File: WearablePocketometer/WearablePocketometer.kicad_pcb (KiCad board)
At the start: 2 copper layers, 66 x 66 mm, 97 parts, among them J101 SolderJumper_2_Bridged, J102 Conn_02x06_Male, J107 SolderJumper_2_Bridged, J111 SolderJumper_2_Bridged, J112 Conn_02x06_Male, J117 SolderJumper_2_Bridged, J120 STANDOFF, J1201 Conn_01x09_Male, J1202 SolderJumper_2_Bridged, J1207 SolderJumper_2_Bridged, J125 STANDOFF, J127 STANDOFF, J129 STANDOFF, J1601 USB_C_Receptacle_USB2.0, J201 SolderJumper_2_Open, J202 Conn_02x06_Male, J207 SolderJumper_2_Open, J701 USB_C_Receptacle_USB2.0, U1001 LSM6DSO, U101 AK09970, U102 P82B96, U104 Teensy4.1, U1101 BME280, U112 P82B96, U1201 AK09970, U1202 P82B96, U1301 LSM6DSO, U1401 BME280, U1501 LSM6DSO, U201 AK09970, U202 P82B96, U301 LSM6DSO, U401 BME280, U501 LSM6DSO, U601 NEO_M8U, U701 USBLC6-2SC6, U801 MIC5319 3.3V, U901 LSM6DSO, Y601 W3011

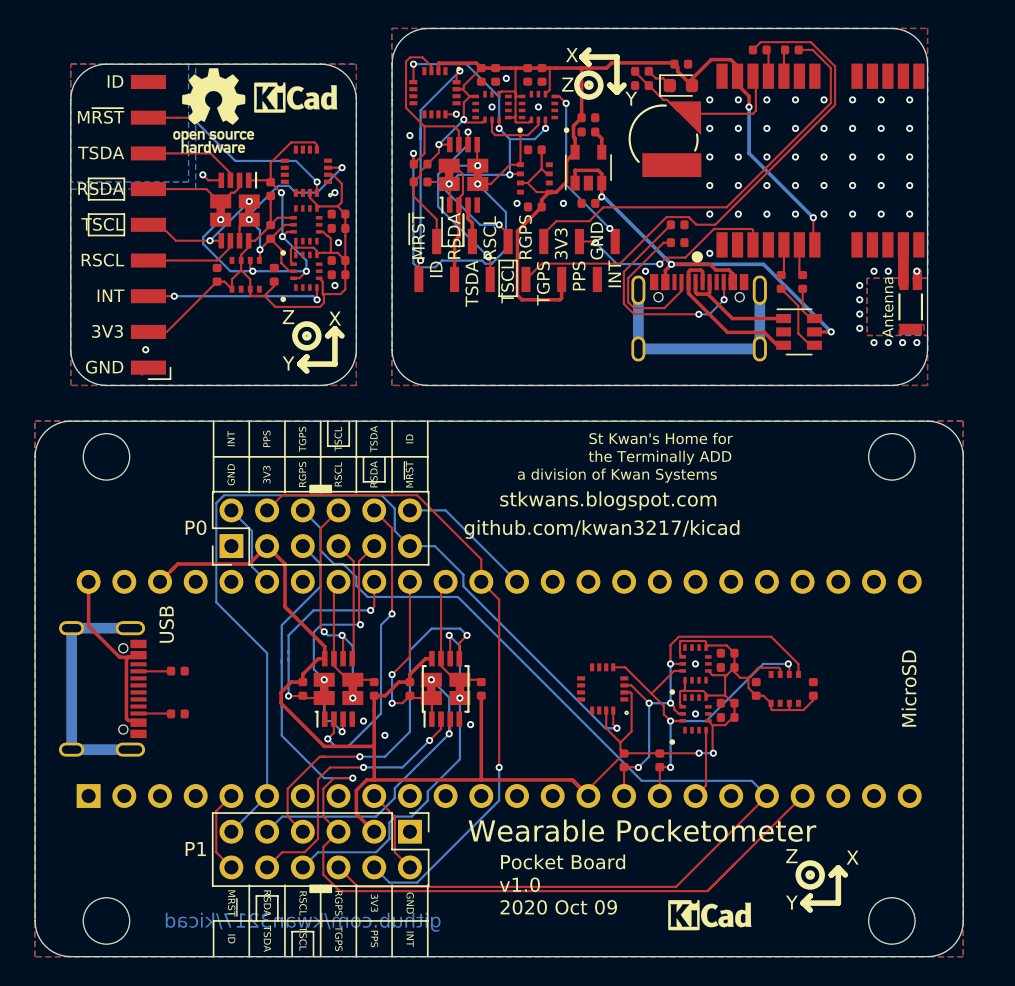
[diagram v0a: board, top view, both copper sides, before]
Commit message: j
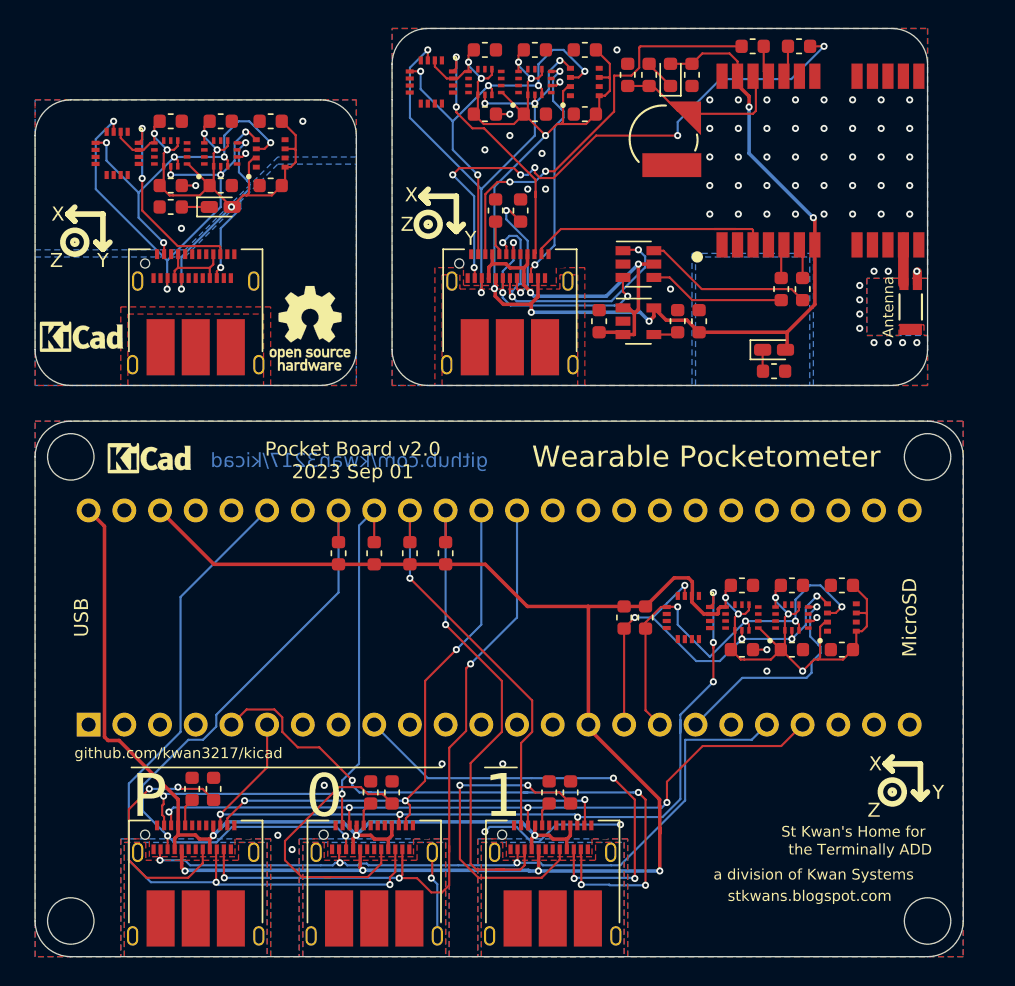
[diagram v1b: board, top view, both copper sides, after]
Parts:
- removed the C801 at (113.0, 73.4)
- removed C804: 100nF, Capacitor_SMD:C_0402_1005Metric
- removed C805: 2.2uF, Capacitor_SMD:C_0402_1005Metric
- removed the G101 at (80.5, 96.3)
- removed the J102 at (100.3, 118.1)
- removed J107, J111, J117, J1202, J1207: SolderJumper_2_Bridged, KwanSystems:SolderJumper-2_Bridged
- removed J112: Conn_02x06_Male, Connector_PinHeader_2.54mm:PinHeader_2x06_P2.54mm_Vertical
- removed J120: STANDOFF, KwanSystems:STANDOFF_NONPLATED
- removed J1601, J701: USB_C_Receptacle_USB2.0, KwanSystems:GCTUSBTypeC_PTH
- removed J201, J207: SolderJumper_2_Open, KwanSystems:SolderJumper-2_Bridged
- removed J202: Conn_02x06_Male, Connector_PinSocket_1.27mm:PinSocket_1x12_P1.27mm_Vertical_SMD_Pin1Left
- removed R1207, R201, R207: 10k, Resistor_SMD:R_0402_1005Metric
- removed R1601, R1602, R701, R702: 5.1k, Resistor_SMD:R_0402_1005Metric
- removed U104: Teensy4.1, KwanSystems:Teensy2x24
- removed U112, U1202, U202: P82B96, Package_SO:TSSOP-8_3x3mm_P0.65mm
- removed the U701 at (128.0, 82.5)
- removed the U801 at (113.0, 70.9)
- added C1001: 1uF, Capacitor_SMD:C_0603_1608Metric, F.Cu at (113.8, 81.8)
- added C1002: 100nF, Capacitor_SMD:C_0603_1608Metric, F.Cu at (119.4, 81.8)
- added C1003: 2.2uF, Capacitor_SMD:C_0603_1608Metric, F.Cu at (120.9, 81.8)
- added D1301: RED, LED_SMD:LED_0603_1608Metric_Castellated, F.Cu at (86.9, 73.7)
- added D501: RED, LED_SMD:LED_0603_1608Metric_Castellated, F.Cu at (126.2, 83.8)
- added J1101: USB_C_Receptacle, KwanSystems:USB_C_Receptacle_Amphenol_12401610E4-2A, F.Cu at (110.5, 122.7)
- added J1701: USB_C_Receptacle, KwanSystems:USB_C_Receptacle_Amphenol_12401610E4-2A, F.Cu at (97.8, 122.7)
- added J1801: USB_C_Receptacle, KwanSystems:USB_C_Receptacle_Amphenol_12401610E4-2A, F.Cu at (85.1, 82.0)
- added J1901: USB_C_Receptacle, KwanSystems:USB_C_Receptacle_Amphenol_12401610E4-2A, F.Cu at (85.1, 122.7)
- added R1101: 5.1k, Resistor_SMD:R_0603_1608Metric, F.Cu at (110.2, 115.3)
- added R1102: 5.1k, Resistor_SMD:R_0603_1608Metric, F.Cu at (111.8, 115.3)
- added R1202: 5.1k, Resistor_SMD:R_0603_1608Metric, F.Cu at (108.2, 73.9)
- added R1301: 1k, Resistor_SMD:R_0603_1608Metric, F.Cu at (83.3, 73.7)
- added R1701: 5.1k, Resistor_SMD:R_0603_1608Metric, F.Cu at (97.5, 115.3)
- added R1702: 5.1k, Resistor_SMD:R_0603_1608Metric, F.Cu at (99.1, 115.3)
- added R1901: 5.1k, Resistor_SMD:R_0603_1608Metric, F.Cu at (84.8, 115.1)
- added R1902: 5.1k, Resistor_SMD:R_0603_1608Metric, F.Cu at (86.4, 115.1)
- added R501: 1k, Resistor_SMD:R_0603_1608Metric, F.Cu at (126.2, 85.3)
- added U1001: MIC5319 3.3V, Package_TO_SOT_SMD:SOT-23-5, F.Cu at (116.6, 81.8)
- added U1201: USBLC6-2SC6, Package_TO_SOT_SMD:SOT-23-6, F.Cu at (116.6, 77.7)
- C1401: renamed from C1305; footprint Capacitor_SMD:C_0402_1005Metric -> Capacitor_SMD:C_0603_1608Metric
- C1402: renamed from C1308; footprint Capacitor_SMD:C_0402_1005Metric -> Capacitor_SMD:C_0603_1608Metric
- C1501: renamed from C1406; footprint Capacitor_SMD:C_0402_1005Metric -> Capacitor_SMD:C_0603_1608Metric
- C1502: renamed from C1408; footprint Capacitor_SMD:C_0402_1005Metric -> Capacitor_SMD:C_0603_1608Metric
- C1601: renamed from C1505; footprint Capacitor_SMD:C_0402_1005Metric -> Capacitor_SMD:C_0603_1608Metric
- C1602: renamed from C1508; footprint Capacitor_SMD:C_0402_1005Metric -> Capacitor_SMD:C_0603_1608Metric
- C201: renamed from C905; footprint Capacitor_SMD:C_0402_1005Metric -> Capacitor_SMD:C_0603_1608Metric
- C202: renamed from C908; footprint Capacitor_SMD:C_0402_1005Metric -> Capacitor_SMD:C_0603_1608Metric
- C301: renamed from C1005; footprint Capacitor_SMD:C_0402_1005Metric -> Capacitor_SMD:C_0603_1608Metric
- C302: renamed from C1008; footprint Capacitor_SMD:C_0402_1005Metric -> Capacitor_SMD:C_0603_1608Metric
- C401: renamed from C1106; footprint Capacitor_SMD:C_0402_1005Metric -> Capacitor_SMD:C_0603_1608Metric
- C402: renamed from C1108; footprint Capacitor_SMD:C_0402_1005Metric -> Capacitor_SMD:C_0603_1608Metric
- C601: renamed from C305; footprint Capacitor_SMD:C_0402_1005Metric -> Capacitor_SMD:C_0603_1608Metric
- C602: renamed from C308; footprint Capacitor_SMD:C_0402_1005Metric -> Capacitor_SMD:C_0603_1608Metric
- C701: renamed from C406; footprint Capacitor_SMD:C_0402_1005Metric -> Capacitor_SMD:C_0603_1608Metric
- C702: renamed from C408; footprint Capacitor_SMD:C_0402_1005Metric -> Capacitor_SMD:C_0603_1608Metric
- C801: renamed from C505; footprint Capacitor_SMD:C_0402_1005Metric -> Capacitor_SMD:C_0603_1608Metric
- C802: renamed from C508; footprint Capacitor_SMD:C_0402_1005Metric -> Capacitor_SMD:C_0603_1608Metric
- C901: renamed from C601; footprint Capacitor_SMD:C_0402_1005Metric -> Capacitor_SMD:C_0603_1608Metric
- G104: renamed from G103; moved to F.Cu
- J101: value SolderJumper_2_Bridged -> STANDOFF; footprint KwanSystems:SolderJumper-2_Bridged -> KwanSystems:STANDOFF_NONPLATED
- J1201: value Conn_01x09_Male -> USB_C_Receptacle; footprint Connector_Harwin:Harwin_M20-89009xx_1x09_P2.54mm_Horizontal -> KwanSystems:USB_C_Receptacle_Amphenol_12401610E4-2A
- R101: renamed from R117; value 10k -> 1k; footprint Resistor_SMD:R_0402_1005Metric -> Resistor_SMD:R_0603_1608Metric
- R102: renamed from R116; value 10k -> 1k; footprint Resistor_SMD:R_0402_1005Metric -> Resistor_SMD:R_0603_1608Metric
- R103: renamed from R141; value 10k -> 1k; footprint Resistor_SMD:R_0402_1005Metric -> Resistor_SMD:R_0603_1608Metric
- R104: renamed from R140; value 10k -> 1k; footprint Resistor_SMD:R_0402_1005Metric -> Resistor_SMD:R_0603_1608Metric
- R105: renamed from R139; value 10k -> 1k; footprint Resistor_SMD:R_0402_1005Metric -> Resistor_SMD:R_0603_1608Metric
- R106: renamed from R138; value 10k -> 1k; footprint Resistor_SMD:R_0402_1005Metric -> Resistor_SMD:R_0603_1608Metric
- R1201: value 10k -> 5.1k; footprint Resistor_SMD:R_0402_1005Metric -> Resistor_SMD:R_0603_1608Metric
- R901: renamed from R605; footprint Resistor_SMD:R_0402_1005Metric -> Resistor_SMD:R_0603_1608Metric
- R902: renamed from R606; footprint Resistor_SMD:R_0402_1005Metric -> Resistor_SMD:R_0603_1608Metric
- R903: renamed from R602; footprint Resistor_SMD:R_0402_1005Metric -> Resistor_SMD:R_0603_1608Metric
- R904: renamed from R603; footprint Resistor_SMD:R_0402_1005Metric -> Resistor_SMD:R_0603_1608Metric
- R905: renamed from R621; footprint Resistor_SMD:R_0402_1005Metric -> Resistor_SMD:R_0603_1608Metric
- R906: renamed from R620; footprint Resistor_SMD:R_0402_1005Metric -> Resistor_SMD:R_0603_1608Metric
- U102: value P82B96 -> Teensy4.1; footprint Package_SO:TSSOP-8_3x3mm_P0.65mm -> KwanSystems:Teensy2x24
- moved G101 51.5 mm to (81.8, 91.4)
- moved G104 38.8 mm to (119.6, 123.7), turned to 0 degrees
- moved J1201 32.0 mm to (107.4, 82.0), turned to 0 degrees
- moved J101 30.5 mm to (76.2, 124.5), turned to 90 degrees
- moved U102 25.5 mm to (77.5, 110.5)
- moved G103 23.3 mm to (122.7, 116.6)
- moved G1301 22.8 mm to (77.0, 82.8)
- moved G502 20.8 mm to (124.7, 81.3)
- moved G504 19.7 mm to (78.5, 74.2), turned to 180 degrees
- moved G1303 16.9 mm to (93.2, 82.3)
- moved R1201 16.1 mm to (106.4, 73.9)
- moved G1304 15.1 mm to (103.6, 72.9)
- moved C1401 14.2 mm to (83.3, 67.6), turned to 0 degrees
- moved G1302 13.9 mm to (92.5, 74.9)
- moved C1601 13.8 mm to (86.9, 67.6), turned to 0 degrees
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- renumbered B601 to B901, D601 to D901, G104 to G102, G102 to G103, G501 to G1301, G502 to G1302, G503 to G1303, G504 to G1304, G901 to G501, G902 to G502, G903 to G503, G904 to G504, J125 to J102, J127 to J103, J129 to J104, U1201 to U1301, U1301 to U1401, U1401 to U1501, U1501 to U1601, U901 to U201, U1001 to U301, U1101 to U401, U201 to U501, U301 to U601, U401 to U701, U501 to U801, U601 to U901, Y601 to Y901
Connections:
- net /Shoe/SCL renamed /Shoe/Q_SCL
- R1201 pad 1: /Shoe/Q_3V3 -> /Shoulder/Shoulder Downstream/CC1
- R1201 pad 2: /Shoe/SDA -> /Shoulder/Q_GND
- R901 pad 1: /Shoulder/GPS/D- -> /Shoulder/D-
- R902 pad 1: /Shoulder/GPS/D+ -> /Shoulder/D+
- U101 pad 1: Net-(U101-Pad1) -> (no net)
- U101 pad 10: Net-(U101-Pad10) -> (no net)
- U101 pad 11: Net-(U101-Pad11) -> (no net)
- U101 pad 14: Net-(U101-Pad14) -> (no net)
- U101 pad 4: Net-(U101-Pad4) -> (no net)
- U101 pad 6: Net-(U101-Pad6) -> (no net)
- U101 pad 7: Net-(U101-Pad7) -> (no net)
- U101 pad 8: Net-(U101-Pad8) -> (no net)
- U101 pad 9: Net-(U101-Pad9) -> (no net)
- U102 pad 1: /P1_SDA -> GND
- U102 pad 2: /P1_TX_SDA -> (no net)
- U102 pad 3: /P1_RX_SDA -> (no net)
- U102 pad 4: GND -> (no net)
- U102 pad 5: /P1_RX_SCL -> /P1_ID
- U102 pad 6: /P1_TX_SCL -> /MAG~RST
- U102 pad 7: /P1_SCL -> (no net)
- U102 pad 8: +3V3 -> (no net)
- U1301 pad 1: Net-(U1201-Pad1) -> (no net)
- U1301 pad 10: Net-(U1201-Pad10) -> (no net)
- U1301 pad 11: Net-(U1201-Pad11) -> (no net)
- U1301 pad 14: Net-(U1201-Pad14) -> (no net)
- U1301 pad 4: Net-(U1201-Pad4) -> (no net)
- U1301 pad 5: /Shoe/SDA -> /Shoe/Q_SDA
- U1301 pad 6: Net-(U1201-Pad6) -> (no net)
- U1301 pad 7: Net-(U1201-Pad7) -> (no net)
- U1301 pad 8: Net-(U1201-Pad8) -> (no net)
- U1301 pad 9: Net-(U1201-Pad9) -> (no net)
- U1401 pad 10: Net-(U1301-Pad10) -> (no net)
- U1401 pad 11: Net-(U1301-Pad11) -> (no net)
- U1401 pad 14: /Shoe/SDA -> /Shoe/Q_SDA
- U1401 pad 9: Net-(U1301-Pad9) -> (no net)
- U1501 pad 3: /Shoe/SDA -> /Shoe/Q_SDA
- U1601 pad 10: Net-(U1501-Pad10) -> (no net)
- U1601 pad 11: Net-(U1501-Pad11) -> (no net)
- U1601 pad 14: /Shoe/SDA -> /Shoe/Q_SDA
- U1601 pad 4: /Shoe/Shoe 6DoF 1/INT -> (no net)
- U1601 pad 9: Net-(U1501-Pad9) -> (no net)
- U201 pad 10: Net-(U901-Pad10) -> (no net)
- U201 pad 11: Net-(U901-Pad11) -> (no net)
- U201 pad 9: Net-(U901-Pad9) -> (no net)
- U301 pad 10: Net-(U1001-Pad10) -> (no net)
- U301 pad 11: Net-(U1001-Pad11) -> (no net)
- U301 pad 4: /Pocket 6DoF 1/INT -> (no net)
- U301 pad 9: Net-(U1001-Pad9) -> (no net)
- U501 pad 1: Net-(U201-Pad1) -> (no net)
- U501 pad 10: Net-(U201-Pad10) -> (no net)
- U501 pad 11: Net-(U201-Pad11) -> (no net)
- U501 pad 14: Net-(U201-Pad14) -> (no net)
- U501 pad 3: /Shoulder/SCL -> /Shoulder/Q_SCL
- U501 pad 4: Net-(U201-Pad4) -> (no net)
- U501 pad 5: /Shoulder/SDA -> /Shoulder/Q_SDA
- U501 pad 6: Net-(U201-Pad6) -> (no net)
- U501 pad 7: Net-(U201-Pad7) -> (no net)
- U501 pad 8: Net-(U201-Pad8) -> (no net)
- U501 pad 9: Net-(U201-Pad9) -> (no net)
- U601 pad 10: Net-(U301-Pad10) -> (no net)
- U601 pad 11: Net-(U301-Pad11) -> (no net)
- U601 pad 13: /Shoulder/SCL -> /Shoulder/Q_SCL
- U601 pad 14: /Shoulder/SDA -> /Shoulder/Q_SDA
- U601 pad 9: Net-(U301-Pad9) -> (no net)
- U701 pad 3: /Shoulder/SDA -> /Shoulder/Q_SDA
- U701 pad 4: /Shoulder/SCL -> /Shoulder/Q_SCL
- U801 pad 10: Net-(U501-Pad10) -> (no net)
- U801 pad 11: Net-(U501-Pad11) -> (no net)
- U801 pad 13: /Shoulder/SCL -> /Shoulder/Q_SCL
- U801 pad 14: /Shoulder/SDA -> /Shoulder/Q_SDA
- U801 pad 4: /Shoulder/Shoulder 6DoF 1/INT -> (no net)
- U801 pad 9: Net-(U501-Pad9) -> (no net)
- U901 pad 1: Net-(U601-Pad1) -> (no net)
- U901 pad 14: Net-(U601-Pad14) -> (no net)
- U901 pad 15: Net-(U601-Pad15) -> (no net)
- U901 pad 16: Net-(U601-Pad16) -> (no net)
- U901 pad 17: Net-(U601-Pad17) -> (no net)
- U901 pad 18: Net-(U601-Pad18) -> (no net)
- U901 pad 19: Net-(U601-Pad19) -> (no net)
- U901 pad 2: Net-(U601-Pad2) -> (no net)
- U901 pad 4: Net-(U601-Pad4) -> (no net)
- U901 pad 8: Net-(U601-Pad8) -> (no net)
- U901 pad 9: Net-(U601-Pad9) -> (no net)
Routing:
- net +5V: track 14.3 -> 68.3 mm, vias 0 -> 3
- net /P0_INT: track 6.13 -> 53.3 mm, vias 0 -> 2
- net /Shoulder/SCL: track 46.8 -> 0.00 mm, vias 2 -> 0
- net /P1_ID: track 5.97 -> 47.1 mm, vias 0 -> 4
- net /P0_ID: track 9.72 -> 49.9 mm, vias 0 -> 3
- net /Shoulder/Q_SCL: track 0.00 -> 38.7 mm, vias 0 -> 5
- net /P0_SCL: track 9.46 -> 48.1 mm, vias 0 -> 2
- net /Shoulder/GPS/SHOULDER_VBUS: track 34.5 -> 0.00 mm, vias 3 -> 0
- net /Shoulder/Q_SDA: track 0.00 -> 31.0 mm, vias 0 -> 5
- net /Shoe/SDA: track 28.3 -> 0.00 mm, vias 5 -> 0
- net /P1_INT: track 6.13 -> 33.3 mm, vias 0 -> 3
- net /P1_SCL: track 9.46 -> 36.4 mm, vias 0 -> 1
- net /Shoulder/SDA: track 26.8 -> 0.00 mm, vias 5 -> 0
- net /P1_TX_SCL: track 26.8 -> 0.00 mm, vias 2 -> 0
- net /P1_RX_SCL: track 26.7 -> 0.00 mm, vias 2 -> 0
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- added copper zone on B.Cu, net Net-(J1101-PadS1)
- added copper zone on F.Cu, net Net-(J1101-PadS1)
- added copper zone on F.Cu, net Net-(J1201-PadS1)
- added copper zone on B.Cu, net Net-(J1701-PadS1)
- added copper zone on F.Cu, net Net-(J1701-PadS1)
- added copper zone on B.Cu, net Net-(J1801-PadS1)
- added copper zone on F.Cu, net Net-(J1801-PadS1)
- added copper zone on B.Cu, net Net-(J1901-PadS1)
- added copper zone on F.Cu, net Net-(J1901-PadS1)
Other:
- outline, holes or cut-outs redrawn
- board text added: "0"
- board text added: "1"
- board text added: "P"
- board text added: "Pocket Board v2.0 2023 Sep 01"
- board text added: "Wearable Pocketometer Shoe Board v2.0 2023 Sep 01"
- board text added: "Wearable Pocketometer Shoulder Board v2.0 2023 Sep 01"
- board text removed: "3V3"
- board text removed: "GND"
- board text removed: "ID"
- board text removed: "INT"
- board text removed: "M~RST"
- board text removed: "P0"
- board text removed: "P1"
- board text removed: "PPS"
- board text removed: "Pocket Board v1.0 2020 Oct 09"
- board text removed: "RGPS"
- board text removed: "RSCL"
- board text removed: "RSDA"
- board text removed: "TGPS"
- board text removed: "TSCL"
- board text removed: "TSDA"
- board text removed: "Wearable Pocketometer Shoe Board v1.0 2020 Sep 01"
- board text removed: "Wearable Pocketometer Shoulder Board v1.0 2020 Sep 01"
